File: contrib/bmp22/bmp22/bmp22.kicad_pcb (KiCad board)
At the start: 2 copper layers, 76 parts, among them J201 Conn_01x10_Male, J202 PH1x4, J301 USB_C_Receptacle_USB2.0, J302 Conn_ARM_JTAG_SWD_10, Q201 DMG1023UV-7, Q202 DMG1024UV-7, Q203 DMG1024UV-7, SW301 SW_DIP_x01, U101 LP2985-3.3, U201 SN74LVC2T45DCUR, U202 SN74LVC2T45DCUR, U203 SN74LVC2T45DCUR, U204 SN74LVC2T45DCUR, U301 USBLC6-2SC6, U302 STM32F103CBUx, Y301 8MHz

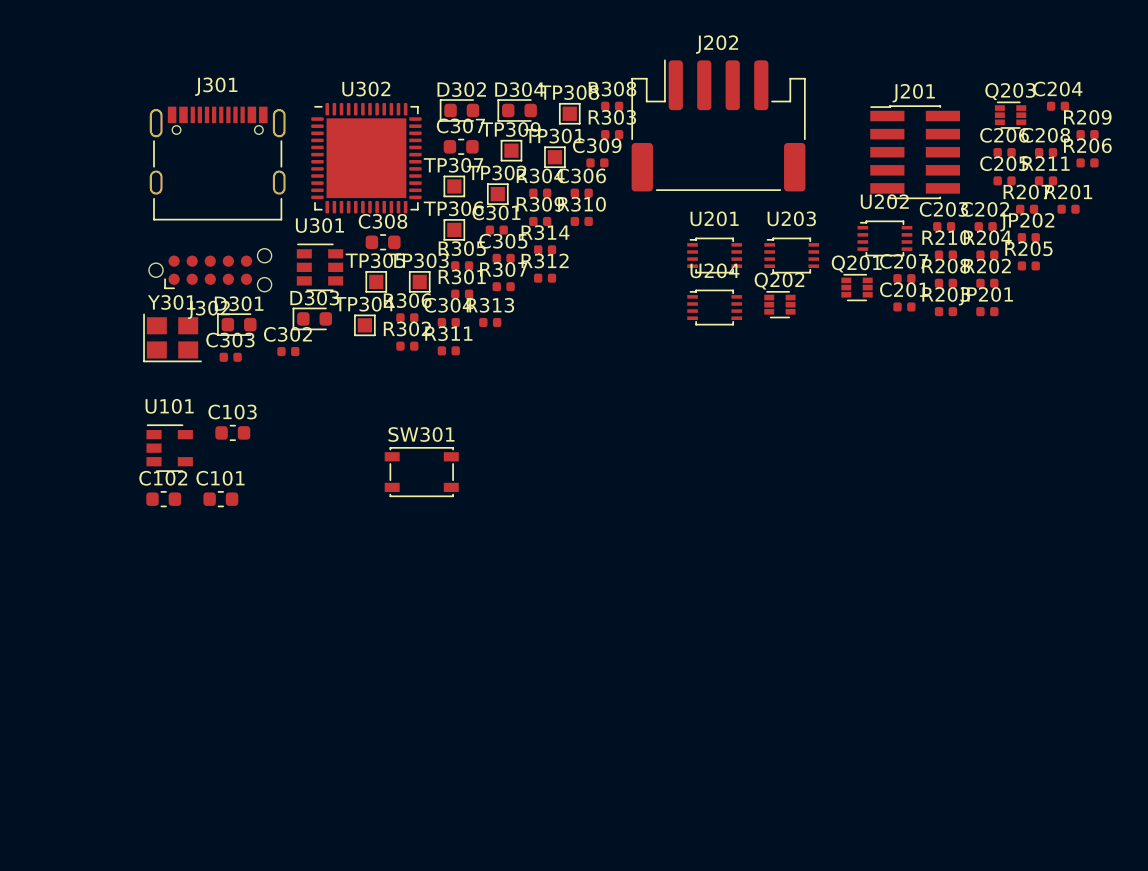
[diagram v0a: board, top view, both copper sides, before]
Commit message: created layout
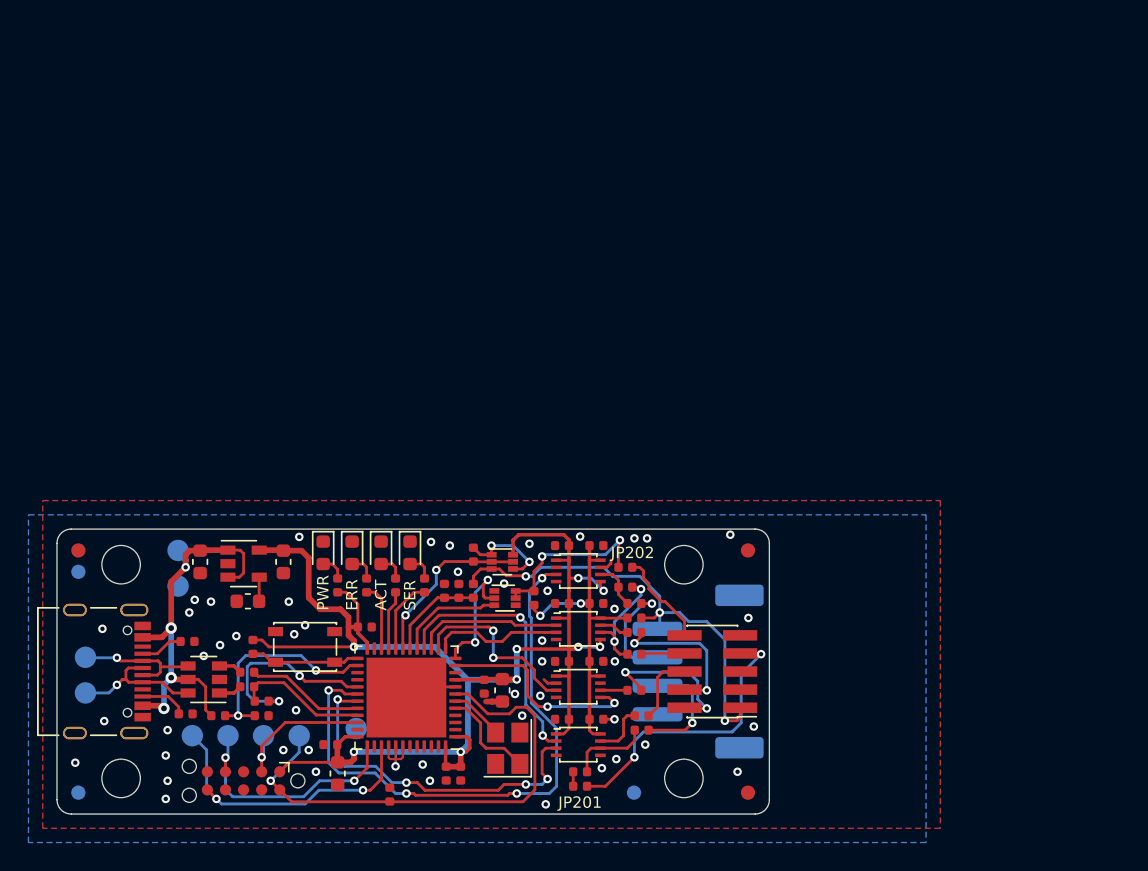
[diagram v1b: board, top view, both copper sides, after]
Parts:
- removed Q202: DMG1024UV-7, Package_TO_SOT_SMD:SOT-563
- added FID1: Fiducial, Fiducial:Fiducial_1mm_Mask2mm, F.Cu at (121.5, 121.5)
- added FID2: Fiducial, Fiducial:Fiducial_1mm_Mask2mm, F.Cu at (168.5, 138.5)
- added FID3: Fiducial, Fiducial:Fiducial_1mm_Mask2mm, F.Cu at (168.5, 121.5)
- added FID4: Fiducial, Fiducial:Fiducial_1mm_Mask2mm, B.Cu at (121.5, 123.0)
- added FID5: Fiducial, Fiducial:Fiducial_1mm_Mask2mm, B.Cu at (160.5, 138.5)
- added FID6: Fiducial, Fiducial:Fiducial_1mm_Mask2mm, B.Cu at (121.5, 138.5)
- added H1: MountingHole, MountingHole:MountingHole_2.7mm_M2.5_DIN965, F.Cu at (124.5, 137.5)
- added H2: MountingHole, MountingHole:MountingHole_2.7mm_M2.5_DIN965, F.Cu at (124.5, 122.5)
- added H3: MountingHole, MountingHole:MountingHole_2.7mm_M2.5_DIN965, F.Cu at (164.0, 137.5)
- added H4: MountingHole, MountingHole:MountingHole_2.7mm_M2.5_DIN965, F.Cu at (164.0, 122.5)
- J202: moved to B.Cu
- TP301, TP302, TP303, TP304, TP305, TP306, TP307, TP309: footprint TestPoint:TestPoint_Pad_1.0x1.0mm -> TestPoint:TestPoint_Pad_D1.5mm; moved to B.Cu
- TP308: value DIO -> SWDIO; footprint TestPoint:TestPoint_Pad_1.0x1.0mm -> TestPoint:TestPoint_Pad_D1.5mm; moved to B.Cu
- moved C204 53.9 mm to (157.9, 133.3)
- moved R209 52.2 mm to (161.0, 134.1), turned to 180 degrees
- moved R308 49.3 mm to (134.4, 133.1)
- moved Q203 49.1 mm to (151.4, 124.8)
- moved TP308 48.7 mm to (134.5, 134.5), turned to 180 degrees
- moved R205 48.2 mm to (156.7, 138.0), turned to 180 degrees
- moved C208 47.7 mm to (157.9, 129.3)
- moved R206 46.9 mm to (160.5, 128.8), turned to 180 degrees
- moved R211 46.4 mm to (153.5, 124.8), turned to 270 degrees
- moved R303 45.6 mm to (133.3, 130.0), turned to 180 degrees
- moved C307 44.8 mm to (139.7, 137.2), turned to 270 degrees
- moved TP301 44.4 mm to (137.0, 134.5), turned to 90 degrees
- moved C203 43.8 mm to (155.4, 133.3), turned to 180 degrees
- moved JP201 43.1 mm to (156.7, 137.0), turned to 180 degrees
- moved C205 42.9 mm to (155.4, 125.2), turned to 180 degrees
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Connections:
- net /Sheet5F25207C/USB+ renamed /Sheet5F25207C/USB_P
- net /Sheet5F25207C/USB- renamed /Sheet5F25207C/USB_N
- D301 pad 1: Net-(D301-Pad1) -> GND
- D301 pad 2: +3V3 -> Net-(D301-Pad2)
- D302 pad 1: Net-(D302-Pad1) -> GND
- D302 pad 2: /Sheet5F25207C/LED0 -> Net-(D302-Pad2)
- D303 pad 1: Net-(D303-Pad1) -> GND
- D303 pad 2: /Sheet5F25207C/LED1 -> Net-(D303-Pad2)
- D304 pad 1: Net-(D304-Pad1) -> GND
- D304 pad 2: /Sheet5F25207C/LED2 -> Net-(D304-Pad2)
- Q201 pad 3: (no net) -> TPWR
- Q201 pad 4: (no net) -> Net-(Q201-Pad1)
- Q201 pad 5: (no net) -> PWR_BR
- R208 pad 2: xRXD -> xTXD
- R209 pad 2: xTXD -> xRXD
- R311 pad 1: Net-(D301-Pad1) -> +3V3
- R311 pad 2: GND -> Net-(D301-Pad2)
- R312 pad 1: Net-(D302-Pad1) -> /Sheet5F25207C/LED0
- R312 pad 2: GND -> Net-(D302-Pad2)
- R313 pad 1: Net-(D303-Pad1) -> /Sheet5F25207C/LED1
- R313 pad 2: GND -> Net-(D303-Pad2)
- R314 pad 1: Net-(D304-Pad1) -> /Sheet5F25207C/LED2
- R314 pad 2: GND -> Net-(D304-Pad2)
- U301 pad 1: /Sheet5F25207C/USBx2- -> /Sheet5F25207C/USBx2+
- U301 pad 3: /Sheet5F25207C/USBx2+ -> /Sheet5F25207C/USBx2-
- U301 pad 4: /Sheet5F25207C/USBx1+ -> /Sheet5F25207C/USBx1-
- U301 pad 6: /Sheet5F25207C/USBx1- -> /Sheet5F25207C/USBx1+
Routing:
- net +3V3: track 0.00 -> 109.0 mm, vias 0 -> 10
- net iTXD: track 0.00 -> 41.3 mm, vias 0 -> 4
- net /Sheet5F25207C/~RST: track 0.00 -> 35.3 mm, vias 0 -> 1
- net TPWR: track 0.00 -> 31.9 mm, vias 0 -> 3
- net +5V: track 0.00 -> 28.6 mm, vias 0 -> 4
- net iRXD: track 0.00 -> 24.8 mm, vias 0 -> 4
- net xTPWR: track 0.00 -> 22.8 mm, vias 0 -> 2
- net /Sheet5F25207C/TRACESWO: track 0.00 -> 20.8 mm, vias 0 -> 2
- net KEY: track 0.00 -> 20.2 mm, vias 0 -> 2
- net iTDO: track 0.00 -> 18.6 mm, vias 0 -> 2
- net /Sheet5F25207C/SWDCLK: track 0.00 -> 17.3 mm, vias 0 -> 2
- net /Sheet5F25207C/VBUS: track 0.00 -> 15.0 mm, vias 0 -> 2
- net iTMS_DIR: track 0.00 -> 14.7 mm, vias 0 -> 2
- net Net-(R309-Pad2): track 0.00 -> 13.6 mm, vias 0 -> 2
- net iTMS: track 0.00 -> 12.8 mm, vias 0 -> 2
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- added copper zone on B.Cu, net GND
- added copper zone on F.Cu, net GND
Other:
- board outline added: 50 x 20 mm
- net class Default: clearance 0.2 -> 0.15; trace_width 0.25 -> 0.2; via_dia 0.8 -> 0.6; via_drill 0.4 -> 0.3
- rule trace_clearance: 0.2 -> 0.15
- rule trace_min: 0.2 -> 0.15
- board text added: "GND"
- board text added: "RXD"
- board text added: "TPWR"
- board text added: "TXD"
